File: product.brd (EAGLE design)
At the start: 59.8 x 31.6 mm, 41 parts, among them IC1 MCP1703CB, Q2 16MHz, U1 ATSHA204-TSU, U2 USB, U3 DISPLAY, U4 TPD4S014_DSQ_10

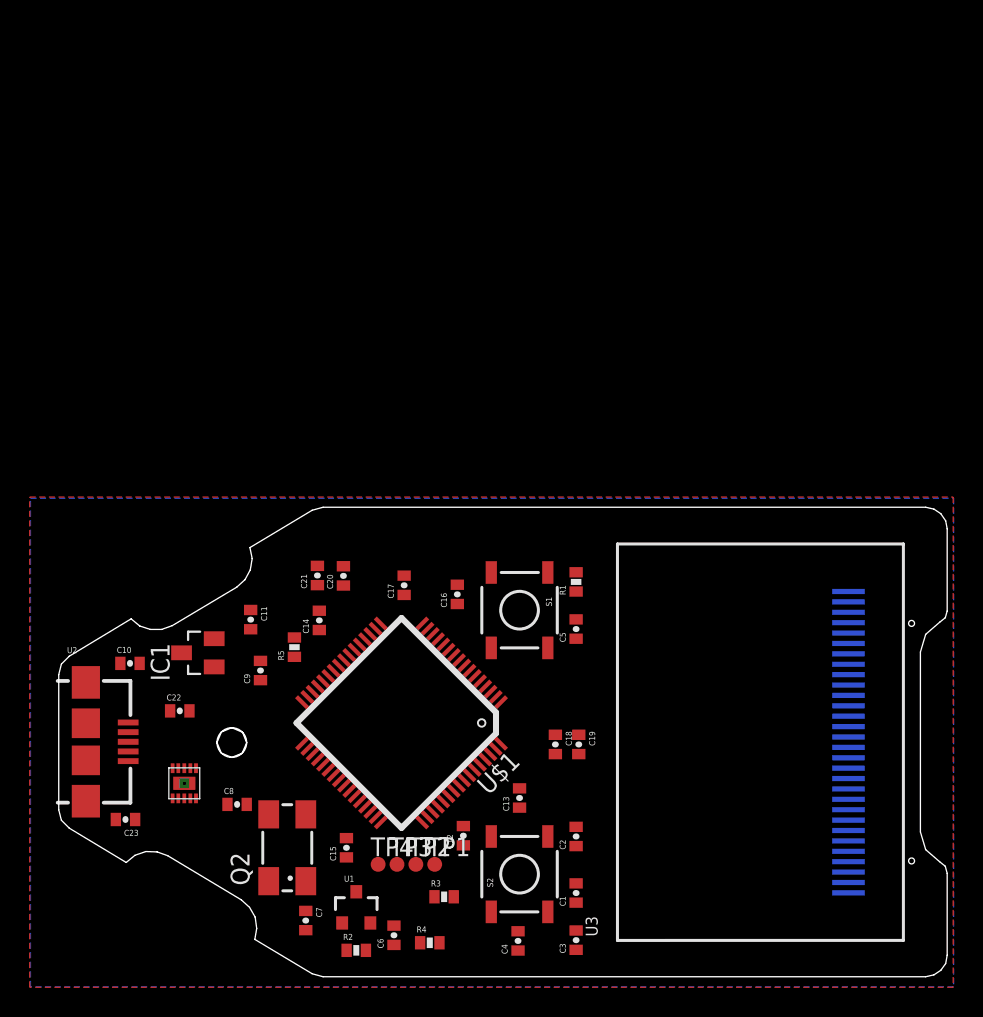
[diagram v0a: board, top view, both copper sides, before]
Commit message: new pcb size :-/
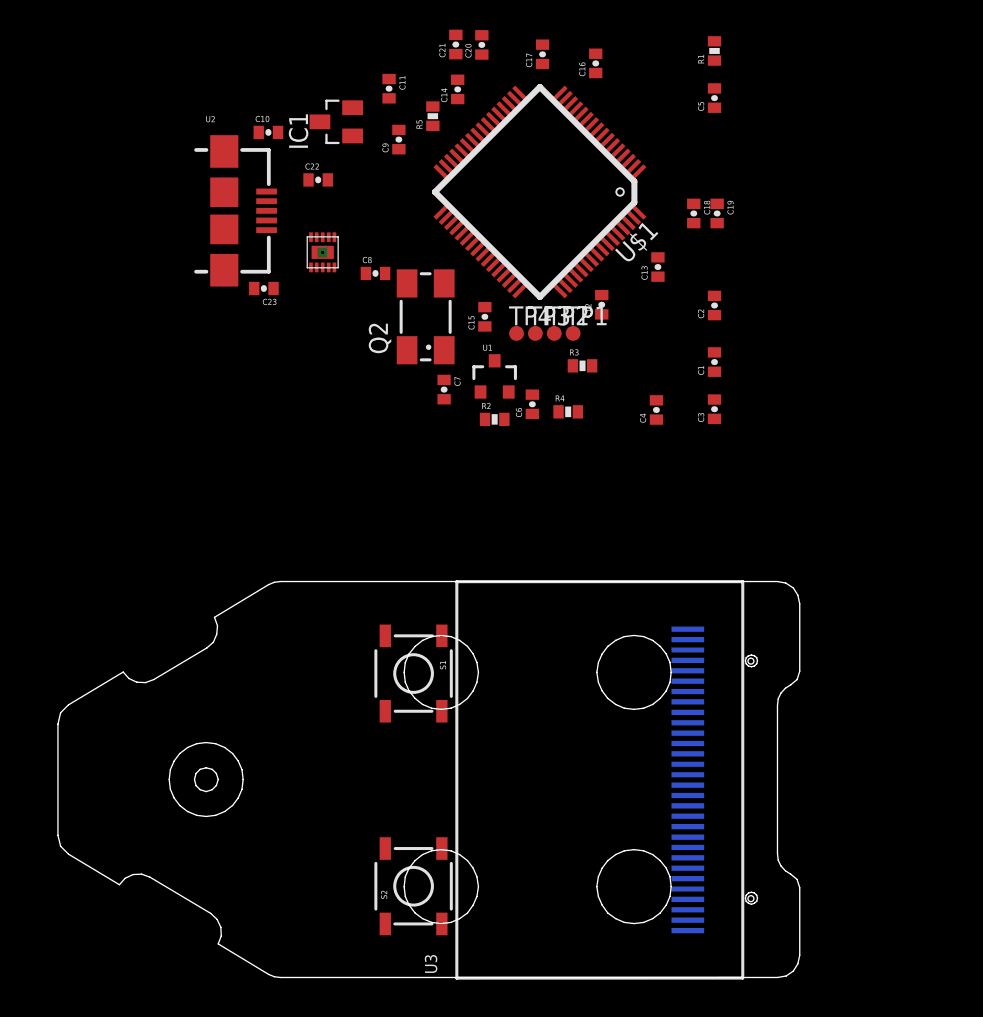
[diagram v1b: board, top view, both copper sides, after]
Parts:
- moved C10 37.0 mm to (14.2, 56.9)
- moved C15 37.0 mm to (28.8, 44.5)
- moved C2 37.0 mm to (44.2, 45.3)
- moved C4 37.0 mm to (40.3, 38.3)
- moved C6 37.0 mm to (32.0, 38.6)
- moved C7 37.0 mm to (26.0, 39.6)
- moved C8 37.0 mm to (21.4, 47.4)
- moved Q2 37.0 mm to (24.8, 44.5)
- moved R2 37.0 mm to (29.4, 37.6)
- moved R3 37.0 mm to (35.4, 41.2)
- moved U1 37.0 mm to (29.4, 40.5)
- moved U2 37.0 mm to (11.2, 51.7)
- moved C1 37.0 mm to (44.2, 41.5)
- moved C11 37.0 mm to (22.3, 59.9)
- moved C12 37.0 mm to (36.7, 45.3)
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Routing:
- removed copper zone on layer 1, net GND
- removed copper zone on layer 16, net GND
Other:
- board size 59.8 x 31.6 mm -> 50 x 26.7 mm
